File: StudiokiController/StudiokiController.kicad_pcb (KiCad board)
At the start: 2 copper layers, 100 x 80 mm, 65 parts, among them J1 USB_B_Mini, J10 Conn_01x30_Male, J2 WJ142R-5.08-3P, J3 Conn_01x04_Female, J4 57PC5FS, J5 Conn_01x02_Female, J6 WJ142R-5.08-3P, J7 WJ142R-5.08-3P, J8 Conn_01x04_Female, J9 Conn_01x04_Female, Q1 Q_DUAL_NPN_NPN_E1B1C2E2B2C1, Q2 PMV20XNE, Q3 PMV20XNE, Q4 PMV20XNE, SW1 SW_Push, SW2 SW_Push, SW3 SW_Push, U1 CH340C, U2 ESP32-WROOM-32D, U3 MAX31855KASA, U4 AZ1117-3.3

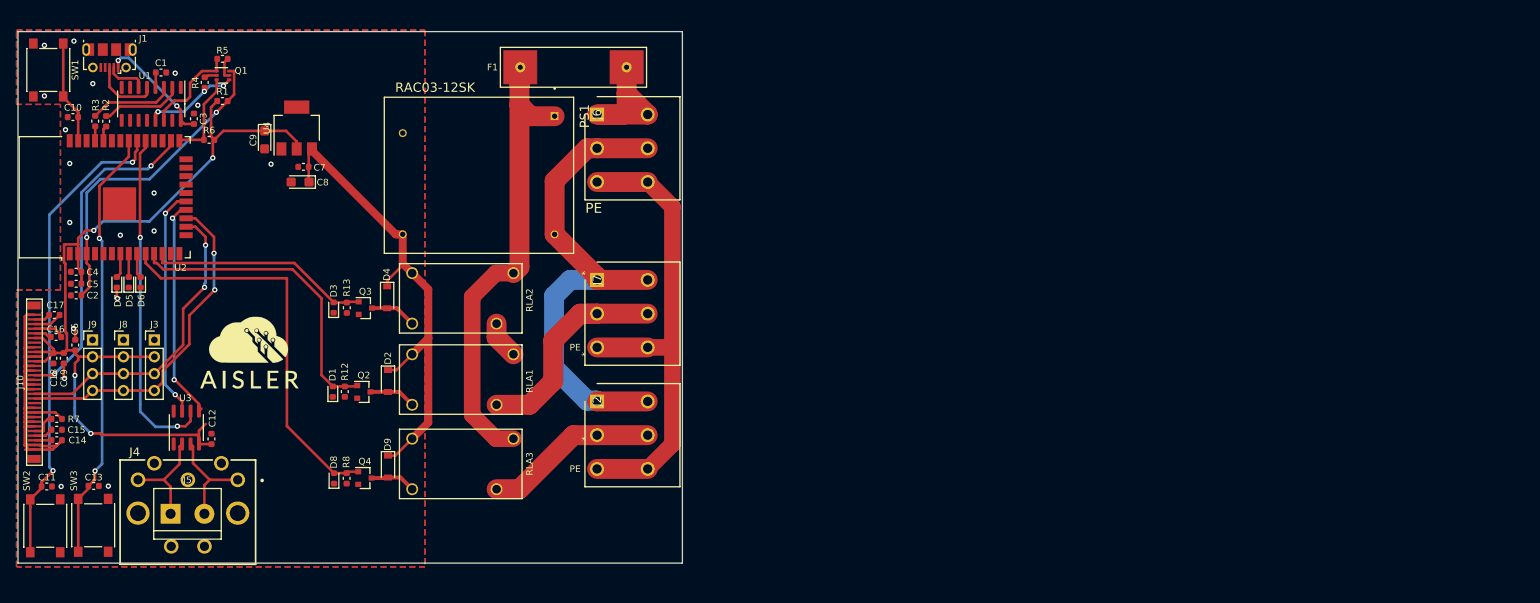
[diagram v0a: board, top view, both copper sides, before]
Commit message: New Layout
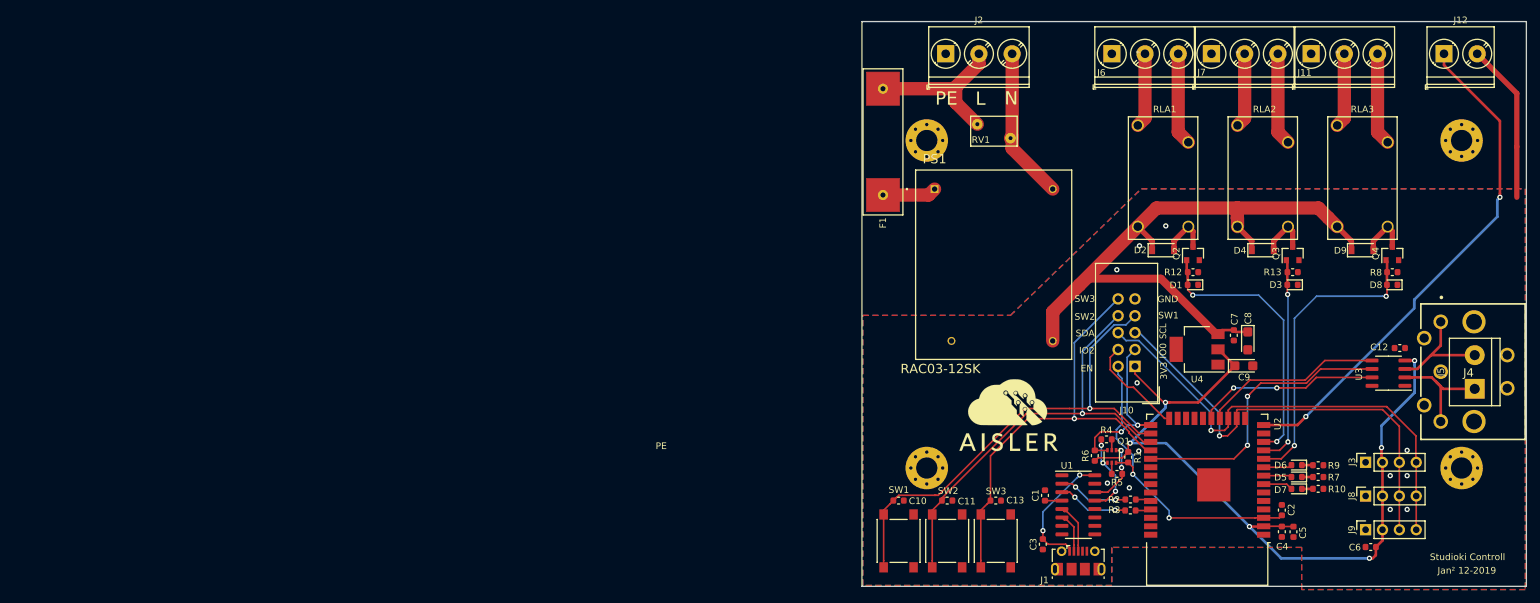
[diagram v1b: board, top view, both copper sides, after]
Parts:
- removed C14: 2.2uF, Capacitor_SMD:C_0603_1608Metric
- removed C15: 4.7uF, Capacitor_SMD:C_0603_1608Metric
- removed C16, C17, C18, C19: 1uF, Capacitor_SMD:C_0603_1608Metric
- added H1: MountingHole, MountingHole:MountingHole_3.2mm_M3_Pad_Via, F.Cu at (186.8, 66.4)
- added H2: MountingHole, MountingHole:MountingHole_3.2mm_M3_Pad_Via, F.Cu at (186.8, 115.7)
- added H3: MountingHole, MountingHole:MountingHole_3.2mm_M3_Pad_Via, F.Cu at (267.3, 66.4)
- added H4: MountingHole, MountingHole:MountingHole_3.2mm_M3_Pad_Via, F.Cu at (267.3, 115.7)
- added J11: Screw_Terminal_01x03, TerminalBlock_Phoenix:TerminalBlock_Phoenix_PT-1,5-3-5.0-H_1x03_P5.00mm_Horizontal, F.Cu at (244.6, 53.3)
- added J12: Screw_Terminal_01x02, TerminalBlock_Phoenix:TerminalBlock_Phoenix_PT-1,5-2-5.0-H_1x02_P5.00mm_Horizontal, F.Cu at (264.6, 53.3)
- added R10: 100, Resistor_SMD:R_0603_1608Metric, F.Cu at (245.7, 118.8)
- added R9: 100, Resistor_SMD:R_0603_1608Metric, F.Cu at (245.7, 115.3)
- added RV1: MOV-07D391KTR, Varistor:RV_Disc_D7mm_W4.5mm_P5mm, F.Cu at (199.4, 66.0)
- J10: value Conn_01x30_Male -> Conn_01x10_Male; footprint StudiokiController:OLED-solder -> Connector_IDC:IDC-Header_2x05_P2.54mm_Vertical
- J2, J6, J7: value WJ142R-5.08-3P -> Screw_Terminal_01x03; footprint StudiokiController:RHDR6W120P762X508_2X3_1524X1410X1355P -> TerminalBlock_Phoenix:TerminalBlock_Phoenix_PT-1,5-3-5.0-H_1x03_P5.00mm_Horizontal
- J3, J8, J9: footprint Connector_PinHeader_2.54mm:PinHeader_1x04_P2.54mm_Vertical -> Connector_PinSocket_2.54mm:PinSocket_1x04_P2.54mm_Vertical
- R7: value 910K -> 100
- moved J4 203.4 mm to (276.9, 101.2), turned to 180 degrees
- moved C6 197.3 mm to (253.6, 127.6), turned to 180 degrees
- moved J5 197.2 mm to (269.3, 103.8), turned to 90 degrees
- moved J9 193.7 mm to (252.8, 125.0), turned to 90 degrees
- moved R7 190.1 mm to (245.7, 117.0), turned to 180 degrees
- moved J8 188.4 mm to (252.8, 119.9), turned to 90 degrees
- moved C5 187.0 mm to (242.0, 125.3), turned to 270 degrees
- moved C4 185.6 mm to (240.2, 125.3), turned to 270 degrees
- moved C2 184.3 mm to (240.2, 122.0), turned to 90 degrees
- moved J3 183.2 mm to (252.8, 114.8), turned to 90 degrees
- moved U3 181.1 mm to (256.3, 101.4), turned to 180 degrees
- moved D7 180.3 mm to (242.5, 118.8), turned to 180 degrees
- moved C12 179.4 mm to (258.0, 97.6), turned to 180 degrees
- moved D5 178.2 mm to (242.5, 117.0), turned to 180 degrees
- moved D6 176.2 mm to (242.5, 115.2), turned to 180 degrees
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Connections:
- D5 pad 1: GND -> Net-(D5-Pad1)
- D6 pad 1: GND -> Net-(D6-Pad1)
- D7 pad 1: GND -> Net-(D7-Pad1)
- J10 pad 1: GND -> +3V3
- J10 pad 10: GND -> SW3
- J10 pad 2: Net-(C17-Pad2) -> EN
- J10 pad 3: Net-(C17-Pad1) -> IO0
- J10 pad 4: Net-(C16-Pad1) -> IO2
- J10 pad 5: Net-(C16-Pad2) -> SCL
- J10 pad 6: +3V3 -> SDA
- J10 pad 7: Net-(J10-Pad7) -> SW1
- J10 pad 8: GND -> SW2
- J10 pad 9: +3V3 -> GND
- J2 pad 1: 230V-N -> PE
- J2 pad 2: 230V-N -> Net-(F1-Pad2)
- J2 pad 3: /sheet5DF376A8/OUTPUT-A -> 230V-N
- J6 pad 1: Net-(F1-Pad2) -> Net-(J6-Pad1)
- J6 pad 2: Net-(F1-Pad2) -> /230V-Relay/OUTPUT-B
- J6 pad 3: 230V-N -> /230V-Relay/OUTPUT-A
- J7 pad 1: 230V-N -> Net-(J7-Pad1)
- J7 pad 2: 230V-N -> /sheet5DF55D65/OUTPUT-B
- J7 pad 3: /230V-Relay/OUTPUT-A -> /sheet5DF55D65/OUTPUT-A
- R7 pad 1: Net-(J10-Pad26) -> GND
- R7 pad 2: GND -> Net-(D5-Pad1)
- RLA1 pad 1: /sheet5DF55D65/OUTPUT-A -> /230V-Relay/OUTPUT-B
- RLA2 pad 1: 230V-L -> /sheet5DF55D65/OUTPUT-B
- RLA3 pad 1: 230V-L -> /sheet5DF376A8/OUTPUT-B
- U2 pad 11: RELAY1 -> RELAY2
- U2 pad 12: RELAY2 -> RELAY1
- U2 pad 14: Net-(U2-Pad14) -> DOOR
- U2 pad 24: Net-(U2-Pad24) -> IO2
- U2 pad 26: DISP_RES -> SW1
- U2 pad 27: Net-(U2-Pad27) -> SW2
- U2 pad 28: Net-(U2-Pad28) -> SW3
- U2 pad 30: SW2 -> Net-(U2-Pad30)
- U2 pad 31: SW3 -> Net-(U2-Pad31)
- U2 pad 37: SW1 -> Net-(U2-Pad37)
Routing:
- net DOOR: track 0.00 -> 77.1 mm, vias 0 -> 2
- net PE: track 73.1 -> 0.00 mm
- net 230V-L: track 70.6 -> 8.20 mm
- net SW1: track 15.6 -> 74.7 mm, vias 0 -> 1
- net 230V-N: track 75.7 -> 23.2 mm
- net DISP_RES: track 49.2 -> 0.00 mm, vias 2 -> 0
- net GND: track 65.4 -> 24.1 mm, vias 18 -> 12
- net +12V: track 74.8 -> 100.5 mm
- net SCL: track 46.6 -> 67.9 mm, vias 2 -> 1
- net SDA: track 50.8 -> 71.4 mm, vias 2 -> 1
- net /230V-Relay/OUTPUT-A: track 33.5 -> 13.9 mm
- net IO2: track 0.00 -> 15.5 mm
- net RELAY3: track 59.7 -> 45.4 mm, vias 0 -> 2
- net +3V3: track 137.3 -> 123.5 mm, vias 4 -> 6
- net IO0: track 13.6 -> 26.8 mm, vias 0 -> 2
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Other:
- board size 100 x 80 mm -> 100 x 85 mm
- board text added: "3V3"
- board text added: "EN"
- board text added: "GND"
- board text added: "IO0"
- board text added: "IO2"
- board text added: "Jan² 12-2019"
- board text added: "L"
- board text added: "N"
- board text added: "SCL"
- board text added: "SDA"
- board text added: "SW1"
- board text added: "SW2"
- board text added: "SW3"
- board text added: "Studioki Controll"
